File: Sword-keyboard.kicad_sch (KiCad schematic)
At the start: 48 parts, among them J1 STX-3000, SW1 SW_Push, SW10 SW_Push, SW11 SW_Push, SW12 SW_Push, SW13 SW_Push, SW14 SW_Push, SW15 SW_Push, SW16 SW_Push, SW17 SW_Push, SW19 SW_Push, SW2 SW_Push, SW20 SW_Push, SW21 SW_Push, SW22 SW_Push, SW23 SW_Push, SW24 SW_Push, SW3 SW_Push, SW4 SW_Push, SW5 SW_Push, SW6 SW_Push, SW7 SW_Push, SW8 SW_Push, SW9 SW_Push, U1 MOUDLE-SEEEDUINO-XIAO

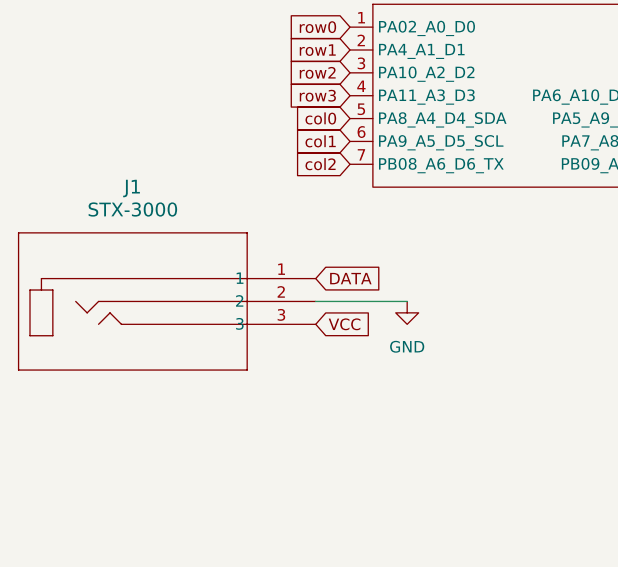
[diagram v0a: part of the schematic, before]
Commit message: Exchanged audio jack
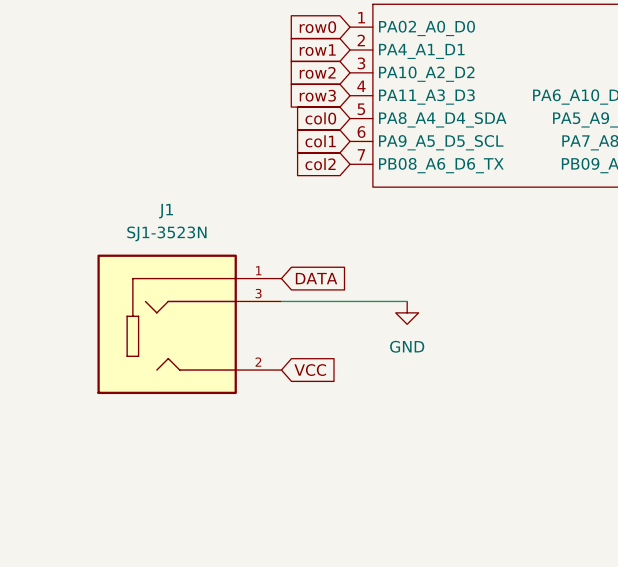
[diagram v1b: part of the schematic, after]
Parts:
- removed J1: STX-3000, STX-3000_KYC, symbol 2024-04-28_16-52-31:STX-3000
- added J1: SJ1-3523N, kicad:CUI_SJ1-3523N, symbol SJ1-3523N:SJ1-3523N
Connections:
- net DATA: now also J1.1
- net GND: now also J1.3
- net VCC: now also J1.2
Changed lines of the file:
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@@
 	(wire
 		(pts
-			(xy 48.26 57.15) (xy 58.42 57.15)
+			(xy 44.45 57.15) (xy 58.42 57.15)
 		)
 		(stroke
@@
 	(global_label "VCC"
 		(shape input)
-		(at 48.26 59.69 0)
+		(at 44.45 64.77 0)
 		(fields_autoplaced yes)
 		(effects
@@
 		)
 		(property "Intersheetrefs" "${INTERSHEET_REFS}"
-			(at 54.8738 59.69 0)
+			(at 51.0638 64.77 0)
 			(effects
 				(font
@@
 	(global_label "DATA"
 		(shape input)
-		(at 48.26 54.61 0)
+		(at 44.45 54.61 0)
 		(fields_autoplaced yes)
 		(effects
@@
 		)
 		(property "Intersheetrefs" "${INTERSHEET_REFS}"
-			(at 55.66 54.61 0)
+			(at 51.85 54.61 0)
 			(effects
 				(font
@@
 	)
 	(symbol
-		(lib_id "2024-04-28_16-52-31:STX-3000")
-		(at 48.26 54.61 0)
-		(unit 1)
-		(exclude_from_sim no)
-		(in_bom yes)
-		(on_board yes)
-		(dnp no)
-		(fields_autoplaced yes)
-		(property "Reference" "J1"
-			(at 27.94 44.45 0)
-			(effects
-				(font
-					(size 1.524 1.524)
-				)
-			)
-		)
-		(property "Value" "STX-3000"
-			(at 27.94 46.99 0)
-			(effects
-				(font
-					(size 1.524 1.524)
-				)
-			)
-		)
-		(property "Footprint" "STX-3000_KYC"
-			(at 48.26 54.61 0)
-			(effects
-				(font
-					(size 1.27 1.27)
-					(italic yes)
-				)
-				(hide yes)
-			)
-		)
-		(property "Datasheet" "STX-3000"
-			(at 48.26 54.61 0)
-			(effects
-				(font
-					(size 1.27 1.27)
-					(italic yes)
-				)
-				(hide yes)
-			)
-		)
-		(property "Description" ""
-			(at 48.26 54.61 0)
-			(effects
-				(font
-					(size 1.27 1.27)
-				)
-				(hide yes)
-			)
-		)
-		(pin "1"
-		)
-		(pin "3"
-		)
-		(pin "2"
-		)
-		(instances
-			(project "Sword-keyboard"
-				(path "/39b32ca6-b7ac-48c3-99e4-87deb7bf18e2"
-					(reference "J1")
-					(unit 1)
-				)
-			)
-		)
-	)
-	(symbol
 		(lib_id "Diode:1N4148")
 		(at 195.58 57.15 90)
@@
 					(unit 1)
 				)
+			)
+		)
+	)
+	(symbol
+		(lib_id "SJ1-3523N:SJ1-3523N")
+		(at 31.75 59.69 0)
+		(unit 1)
+		(exclude_from_sim no)
+		(in_bom yes)
+		(on_board yes)
+		(dnp no)
+		(fields_autoplaced yes)
+		(property "Reference" "J1"
+			(at 31.75 46.99 0)
+			(effects
+				(font
+					(size 1.27 1.27)
+				)
+			)
+		)
+		(property "Value" "SJ1-3523N"
+			(at 31.75 49.53 0)
+			(effects
+				(font
+					(size 1.27 1.27)
+				)
+			)
+		)
+		(property "Footprint" "kicad:CUI_SJ1-3523N"
+			(at 31.75 59.69 0)
+			(effects
+				(font
+					(size 1.27 1.27)
+				)
+				(justify bottom)
+				(hide yes)
+			)
+		)
+		(property "Datasheet" ""
+			(at 31.75 59.69 0)
+			(effects
+				(font
+					(size 1.27 1.27)
+				)
+				(hide yes)
+			)
+		)
+		(property "Description" ""
+			(at 31.75 59.69 0)
+			(effects
+				(font
+					(size 1.27 1.27)
+				)
+				(hide yes)
+			)
+		)
+		(property "PARTREV" "1.05"
+			(at 31.75 59.69 0)
+			(effects
+				(font
+					(size 1.27 1.27)
+				)
+				(justify bottom)
+				(hide yes)
+			)
+		)
+		(property "STANDARD" "Manufacturer Recommendations"
+			(at 31.75 59.69 0)
+			(effects
+				(font
+					(size 1.27 1.27)
+				)
+				(justify bottom)
+				(hide yes)
+			)
+		)
+		(property "MAXIMUM_PACKAGE_HEIGHT" "6.25 mm"
+			(at 31.75 59.69 0)
+			(effects
+				(font
+					(size 1.27 1.27)
+				)
+				(justify bottom)
+				(hide yes)
+			)
+		)
+		(property "MANUFACTURER" "CUI Devices"
+			(at 31.75 59.69 0)
+			(effects
+				(font
+					(size 1.27 1.27)
+				)
+				(justify bottom)
+				(hide yes)
+			)
+		)
+		(pin "2"
+		)
+		(pin "1"
+		)
+		(pin "3"
+		)
+		(instances
+			(project "Sword-keyboard"
+				(path "/39b32ca6-b7ac-48c3-99e4-87deb7bf18e2"
+					(reference "J1")
+					(unit 1)
+				)
